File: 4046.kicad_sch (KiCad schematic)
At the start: 10 parts, among them SW6 PLL Type, U9 4046

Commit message: start smd refactoring
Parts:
- C4, C5: footprint Capacitor_THT:C_Disc_D4.3mm_W1.9mm_P5.00mm -> C_0805_2012Metric; KiLib_Generator (none) -> SMD_2terminal_chip_molded
- C6: footprint Capacitor_THT:C_Disc_D5.0mm_W2.5mm_P5.00mm -> C_0805_2012Metric; KiLib_Generator (none) -> SMD_2terminal_chip_molded
- R27, R28: footprint Resistor_THT:R_Axial_DIN0207_L6.3mm_D2.5mm_P10.16mm_Horizontal -> R_0805_2012Metric; KiLib_Generator (none) -> SMD_2terminal_chip_molded
- SW6: footprint Button_Switch_THT:SW_E-Switch_EG1271_SPDT -> SW_SPDT_CK_JS102011SAQN
- U9: footprint Package_DIP:DIP-16_W7.62mm -> SOIC-16_3.9x9.9mm_P1.27mm; KiLib_Generator (none) -> package/gullwing
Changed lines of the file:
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@@
 			)
 		)
-		(property "Footprint" "Capacitor_THT:C_Disc_D4.3mm_W1.9mm_P5.00mm"
+		(property "Footprint" "C_0805_2012Metric"
 			(at 119.38 63.1952 0)
 			(hide yes)
@@
 			)
 		)
-		(property "Description" "Unpolarized capacitor"
+		(property "Description" ""
+			(at 123.19 62.23 0)
+			(hide yes)
+			(show_name no)
+			(do_not_autoplace no)
+			(effects
+				(font
+					(size 1.27 1.27)
+				)
+			)
+		)
+		(property "KiLib_Generator" "SMD_2terminal_chip_molded"
 			(at 123.19 62.23 0)
 			(hide yes)
@@
 			)
 		)
-		(property "Footprint" "Button_Switch_THT:SW_E-Switch_EG1271_SPDT"
+		(property "Footprint" "SW_SPDT_CK_JS102011SAQN"
 			(at 181.61 64.77 0)
 			(hide yes)
@@
 			)
 		)
-		(property "Description" "Switch, single pole double throw"
+		(property "Description" ""
 			(at 181.61 64.77 0)
 			(hide yes)
@@
 			)
 		)
-		(property "Footprint" "Package_DIP:DIP-16_W7.62mm"
+		(property "Footprint" "SOIC-16_3.9x9.9mm_P1.27mm"
 			(at 152.4 69.85 0)
 			(hide yes)
@@
 			)
 		)
-		(property "Datasheet" "https://assets.nexperia.com/documents/data-sheet/HEF4046B.pdf"
+		(property "Datasheet" ""
 			(at 152.4 69.85 0)
 			(hide yes)
@@
 			)
 		)
-		(property "Description" "Phase Comp & VCO"
+		(property "Description" ""
+			(at 152.4 69.85 0)
+			(hide yes)
+			(show_name no)
+			(do_not_autoplace no)
+			(effects
+				(font
+					(size 1.27 1.27)
+				)
+			)
+		)
+		(property "KiLib_Generator" "package/gullwing"
 			(at 152.4 69.85 0)
 			(hide yes)
@@
 			)
 		)
-		(property "Footprint" "Resistor_THT:R_Axial_DIN0207_L6.3mm_D2.5mm_P10.16mm_Horizontal"
+		(property "Footprint" "R_0805_2012Metric"
 			(at 128.27 99.06 0)
 			(hide yes)
@@
 			)
 		)
-		(property "Description" "Resistor, small symbol"
+		(property "Description" ""
+			(at 128.27 99.06 0)
+			(hide yes)
+			(show_name no)
+			(do_not_autoplace no)
+			(effects
+				(font
+					(size 1.27 1.27)
+				)
+			)
+		)
+		(property "KiLib_Generator" "SMD_2terminal_chip_molded"
 			(at 128.27 99.06 0)
 			(hide yes)
@@
 			)
 		)
-		(property "Footprint" "Resistor_THT:R_Axial_DIN0207_L6.3mm_D2.5mm_P10.16mm_Horizontal"
+		(property "Footprint" "R_0805_2012Metric"
 			(at 139.7 99.06 0)
 			(hide yes)
@@
 			)
 		)
-		(property "Description" "Resistor, small symbol"
+		(property "Description" ""
+			(at 139.7 99.06 0)
+			(hide yes)
+			(show_name no)
+			(do_not_autoplace no)
+			(effects
+				(font
+					(size 1.27 1.27)
+				)
+			)
+		)
+		(property "KiLib_Generator" "SMD_2terminal_chip_molded"
 			(at 139.7 99.06 0)
 			(hide yes)
@@
 			)
 		)
-		(property "Footprint" "Capacitor_THT:C_Disc_D5.0mm_W2.5mm_P5.00mm"
+		(property "Footprint" "C_0805_2012Metric"
 			(at 185.7248 85.09 0)
 			(hide yes)
@@
 			)
 		)
-		(property "Description" "Unpolarized capacitor"
+		(property "Description" ""
+			(at 186.69 88.9 0)
+			(hide yes)
+			(show_name no)
+			(do_not_autoplace no)
+			(effects
+				(font
+					(size 1.27 1.27)
+				)
+			)
+		)
+		(property "KiLib_Generator" "SMD_2terminal_chip_molded"
 			(at 186.69 88.9 0)
 			(hide yes)
@@
 			)
 		)
-		(property "Footprint" "Capacitor_THT:C_Disc_D4.3mm_W1.9mm_P5.00mm"
+		(property "Footprint" "C_0805_2012Metric"
 			(at 132.08 68.58 0)
 			(hide yes)
@@
 			)
 		)
-		(property "Description" "Unpolarized capacitor, small symbol"
+		(property "Description" ""
 			(at 132.08 68.58 0)
 			(hide yes)
+			(show_name no)
+			(do_not_autoplace no)
+			(effects
+				(font
+					(size 1.27 1.27)
+				)
+			)
+		)
+		(property "KiLib_Generator" "SMD_2terminal_chip_molded"
+			(at 132.08 68.58 0)
+			(hide yes)

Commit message: back to kicad 10.0
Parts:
- SW6: footprint SW_SPDT_CK_JS102011SAQN -> Button_Switch_THT:SW_Slide_SPDT_Straight_CK_OS102011MS2Q
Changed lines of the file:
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@@
 (kicad_sch
-	(version 20260826)
+	(version 20260306)
 	(generator "eeschema")
-	(generator_version "10.99")
+	(generator_version "10.0")
 	(paper "A4")
 	(junction
@@
 			)
 		)
-		(property "Footprint" "SW_SPDT_CK_JS102011SAQN"
+		(property "Footprint" "Button_Switch_THT:SW_Slide_SPDT_Straight_CK_OS102011MS2Q"
 			(at 181.61 64.77 0)
 			(hide yes)

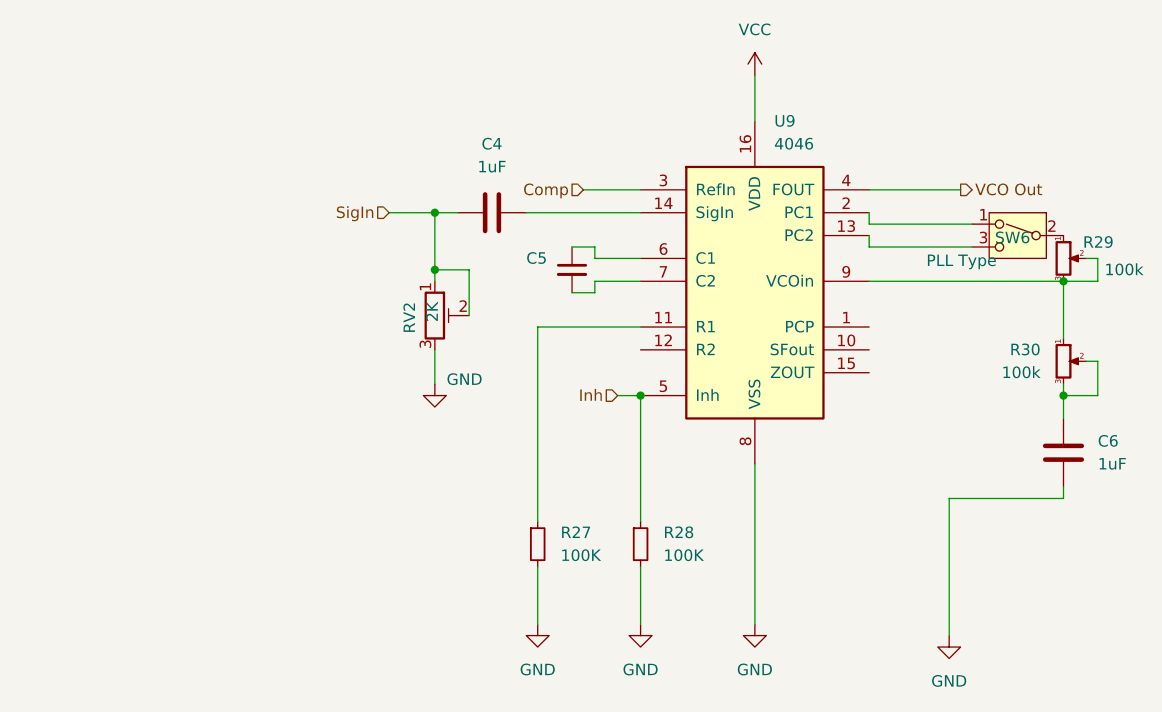
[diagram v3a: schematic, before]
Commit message: wip rerouting
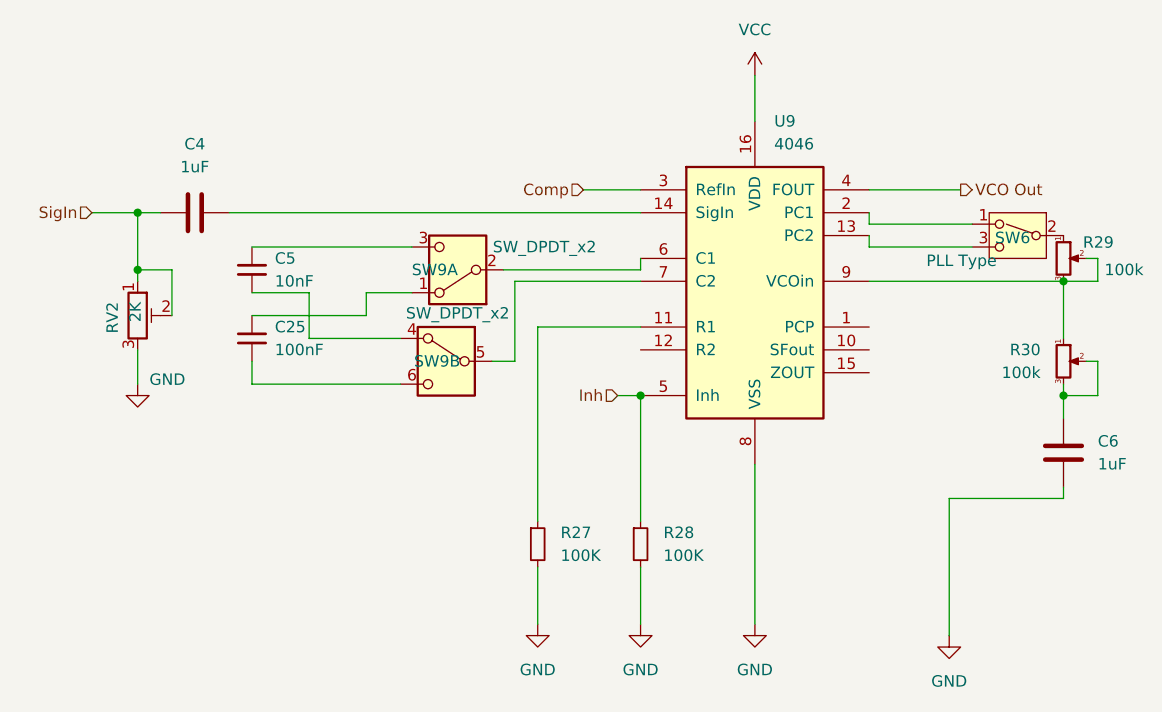
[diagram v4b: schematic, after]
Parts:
- added C25: 100nF, Capacitor_SMD:C_0805_2012Metric, symbol Device:C_Small
- added SW9: SW_DPDT_x2, Button_Switch_THT:SW_CK_JS202011CQN_DPDT_Straight, symbol Switch:SW_DPDT_x2
- C5: value C1 -> 10nF; footprint C_0805_2012Metric -> Capacitor_SMD:C_0805_2012Metric; KiLib_Generator SMD_2terminal_chip_molded -> (none)
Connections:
- net at U9.6 (C1): now also SW9.2 (B); no longer C5.1
- net at U9.7 (C2): now also SW9.5 (B); no longer C5.2
- new net: C25.1, SW9.1 (A)
- new net: C5.1, SW9.3 (C)
- new net: C5.2, SW9.4 (A)
- new net: C25.2, SW9.6 (C)
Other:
- moved on the sheet: C4, RV2
